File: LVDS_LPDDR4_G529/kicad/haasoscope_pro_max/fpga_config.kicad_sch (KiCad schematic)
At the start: 1 part, among them U3 Ti90G529_Functions

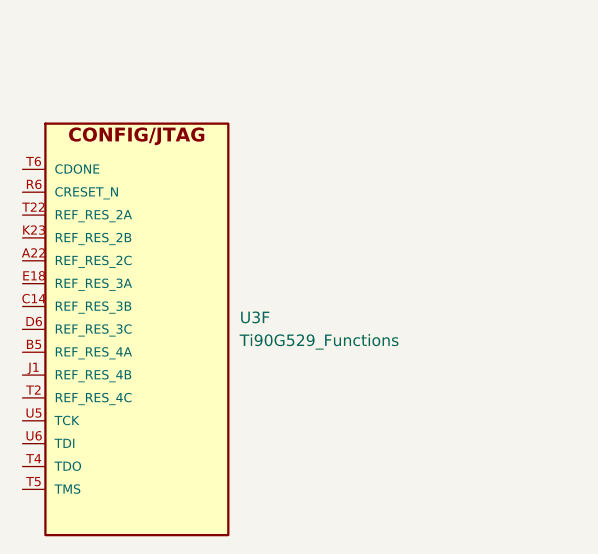
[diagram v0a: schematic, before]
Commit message: Aligned schematics, sort of
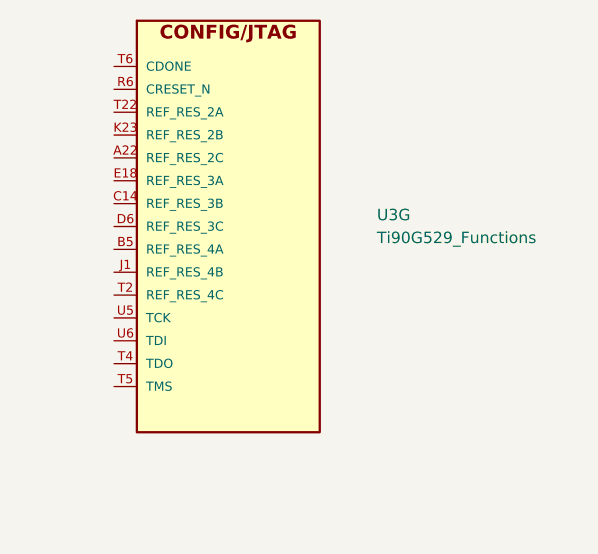
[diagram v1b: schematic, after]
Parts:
- removed U3: Ti90G529_Functions, G529:BGA-529_23x23_19.0x19.0mm, symbol Ti90G529_Functions:Ti90G529_Functions
- added U3: Ti90G529_Functions, haasoscope_pro_adc_fpga_board:BGA-529_23x23_19.0x19.0mm, symbol Ti90G529_Functions:Ti90G529_Functions
